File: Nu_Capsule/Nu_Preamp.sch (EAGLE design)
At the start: 20 parts, among them T1 2SC3324, T2 2SC3324

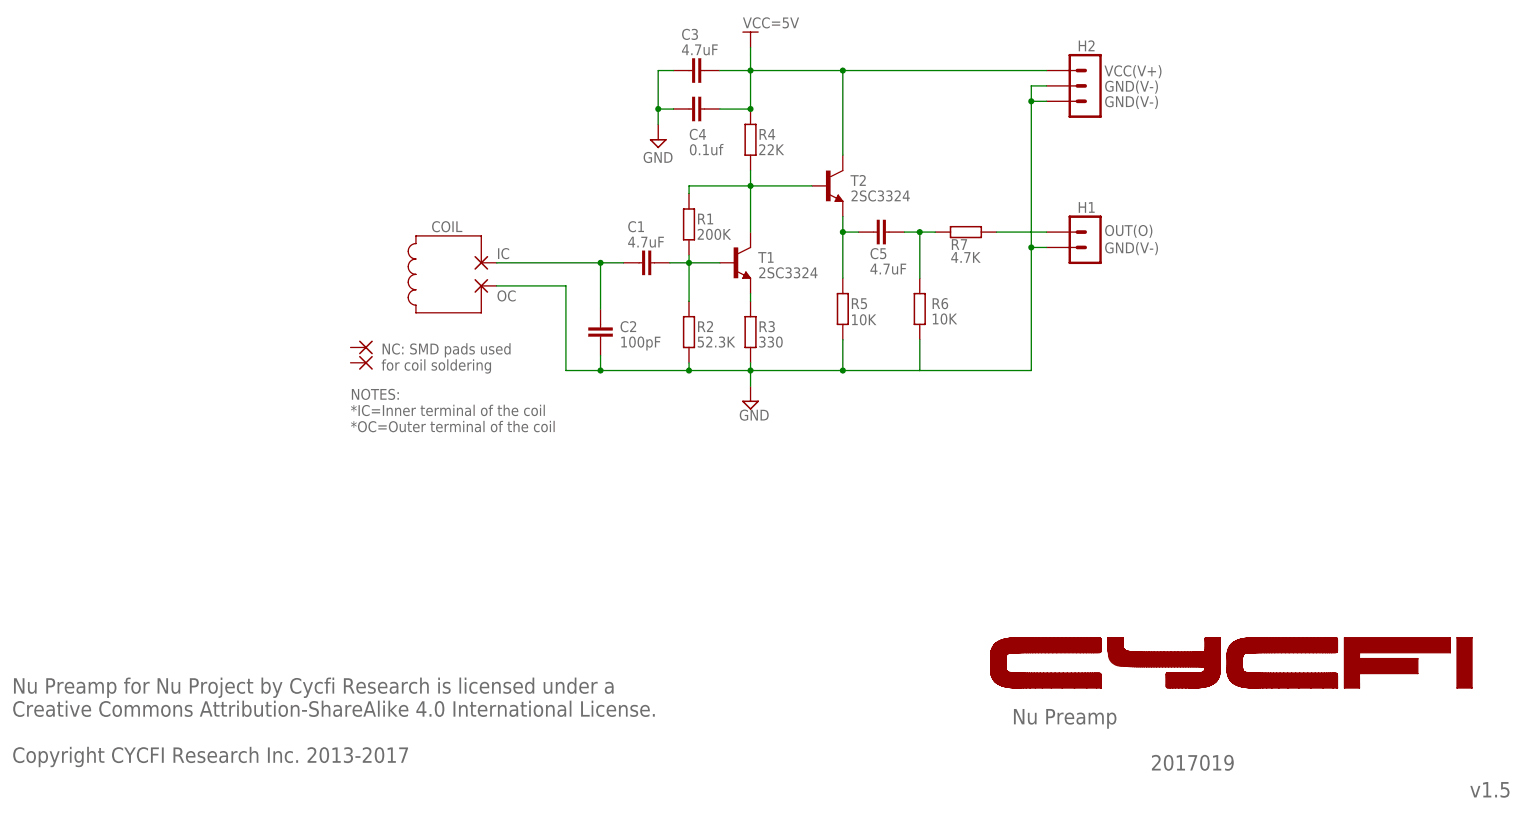
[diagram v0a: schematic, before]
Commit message: Updated files for version 2.0
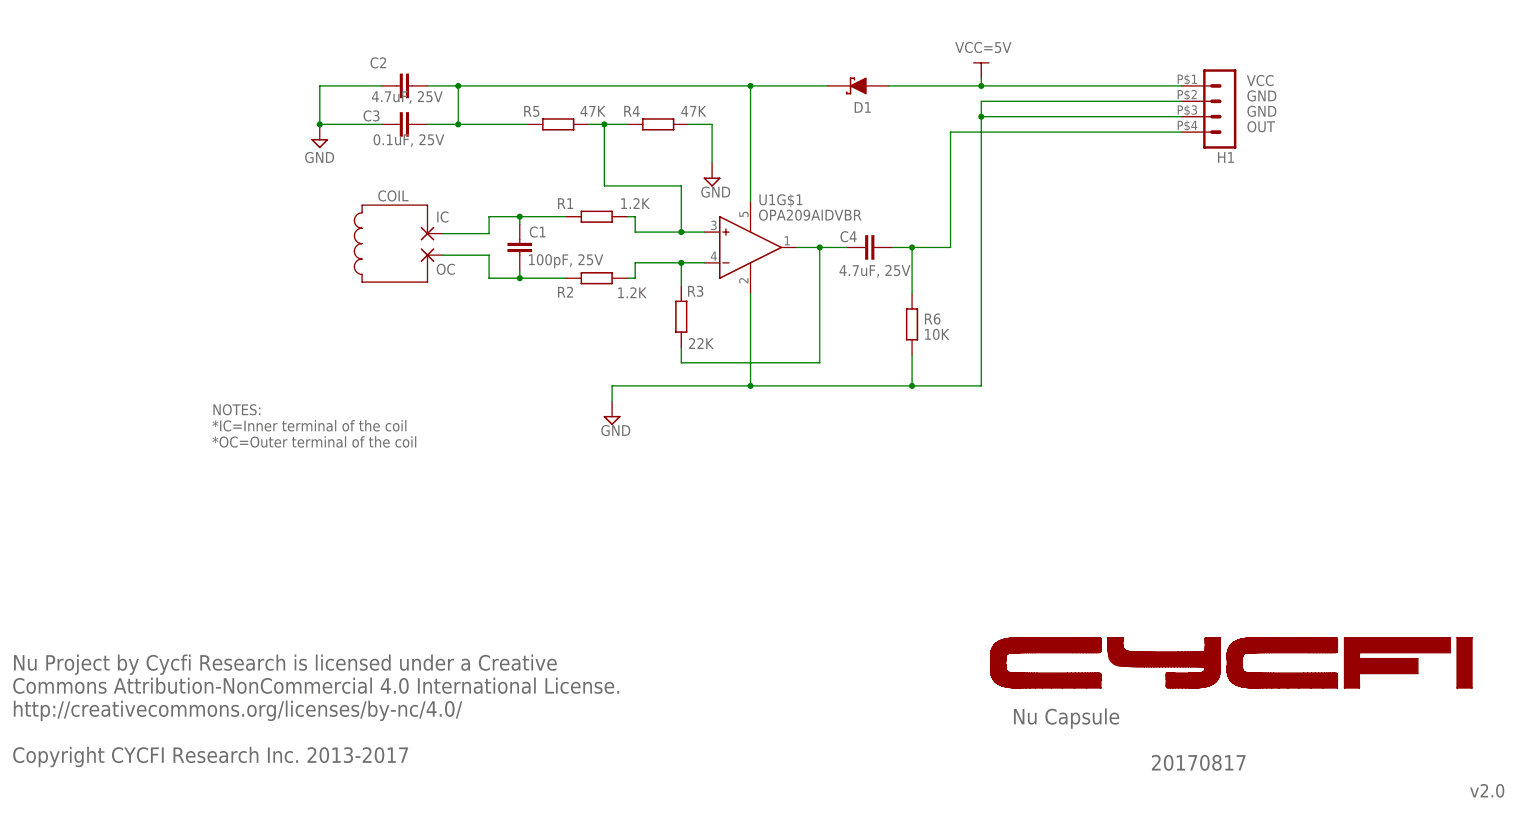
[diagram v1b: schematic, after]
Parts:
- removed C5: 4.7uF, resistor:C-EUC0603
- removed H2: 3P-2MM-TH-MALE, CYCFI_Con:3P-2MM-TH-MALE
- removed PAD18, PAD19, PAD6, PAD7: WIREPADSMD1,27-254, wirepad:WIREPADSMD1,27-254
- removed R7: 4.7K, resistor:R-EU_R0402
- removed T1, T2: 2SC3324, transistor:BC846
- added D1: (no value), m-pad-2.1:D_SCHOTTKYL
- added IC, OC: (no value), wirepad:1,6/0,8
- added U1: OPA209AIDVBR, CYCFI_semicon:OPA209DBVR
- C1: value 4.7uF -> 100pF, 25V; device resistor:C-EUC0603 -> rcl:C-EUC0402
- C2: value 100pF -> 4.7uF, 25V; device resistor:C-EUC0603 -> rcl:C0603_NK
- C3: value 4.7uF -> 0.1uF, 25V; device resistor:C-EUC0603 -> rcl:C-EUC0402
- C4: value 0.1uf -> 4.7uF, 25V; device resistor:C-EUC0603 -> rcl:C-EUC0603
- H1: value 2P-2MM-TH-MALE -> 4P_ZIF_59453-041110EDHLF; device CYCFI_Con:2P-2MM-TH-MALE -> CYCFI_Con:4P_ZIF_59453-041110EDHLF
- R1: value 200K -> 1.2K; device resistor:R-EU_R0603 -> resistor:R-EU_R0402
- R2: value 52.3K -> 1.2K
- R3: value 330 -> 22K
- R4: value 22K -> 47K
- R5: value 10K -> 47K
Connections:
- removed net N$3: C5.2, R5.2, T2.E
- removed net OUTPUT: H1.1, R7.2
- removed net VCVF: R1.2, R4.1, T1.C, T2.B
- removed net VIN: C3.2, C4.2, H2.1, R4.2, T2.C
- new net N$5: C4.1, R3.2, U1G$1.OUT
- new net N$6: R1.2, R4.1, R5.2, U1G$1.IN+
- new net N$7: R2.2, R3.1, U1G$1.IN-
- new net VCC: C2.2, C3.2, D1.C, R5.1, U1G$2.V+
- net GND: now also H1.3, R4.2, U1G$2.V-; no longer C4.1, H2.2, H2.3, PAD7.P, R2.1, R3.1, R5.1
- net N$1: now also D1.A, H1.1; no longer C1.2, R1.1, R2.2, T1.B
- net N$2: now also IC.P, R1.1; no longer C2.2, PAD6.P
- net N$4: now also C1.2, OC.P, R2.1; no longer R3.2, T1.E
- net OUT: now also C4.2, H1.4; no longer C5.1, R7.1
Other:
- note added: "20170817"
- note added: "GND"
- note added: "Nu Capsule"
- note added: "Nu Project by Cycfi Research is licensed under a Creative Commons Attribution-NonCommercial 4.0 International License. http://creativecommons.org/licenses/by-nc/4.0/ Copyright CYCFI Research Inc. 2013-2017"
- note added: "OUT"
- note added: "VCC"
- note added: "v2.0"
- note removed: "2017019"
- note removed: "GND(V-)"
- note removed: "IC"
- note removed: "NC: SMD pads used for coil soldering"
- note removed: "Nu Preamp"
- note removed: "Nu Preamp for Nu Project by Cycfi Research is licensed under a Creative Commons Attribution-ShareAlike 4.0 International License. Copyright CYCFI Research Inc. 2013-2017"
- note removed: "OC"
- note removed: "OUT(O)"
- note removed: "VCC(V+)"
- note removed: "v1.5"
- moved on the sheet: C1, C2, C3, C4, R1, R2, R3, R4, R5, R6
